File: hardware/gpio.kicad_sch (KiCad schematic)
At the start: 23 parts, among them J2 HDMI_C_1.3, U3 ECP5U_12_CABGA256, U5 PCA9306DC1

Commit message: Add a revision
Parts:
- R16, R18: JLCPCB Part # C25117 -> C25117
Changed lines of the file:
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@@
 			)
 		)
-		(property "JLCPCB Part #" "C25117 "
+		(property "JLCPCB Part #" "C25117"
 			(at 184.15 109.22 0)
 			(effects
@@
 			)
 		)
-		(property "JLCPCB Part #" "C25117 "
+		(property "JLCPCB Part #" "C25117"
 			(at 184.15 93.98 0)
 			(effects

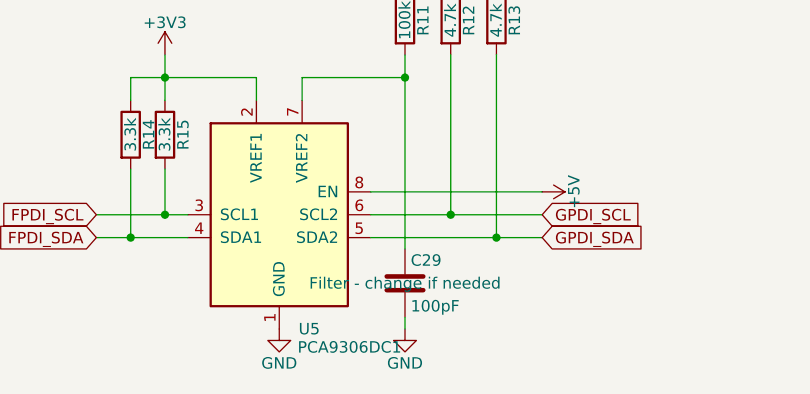
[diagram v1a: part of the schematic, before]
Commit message: Pre-prod fixes
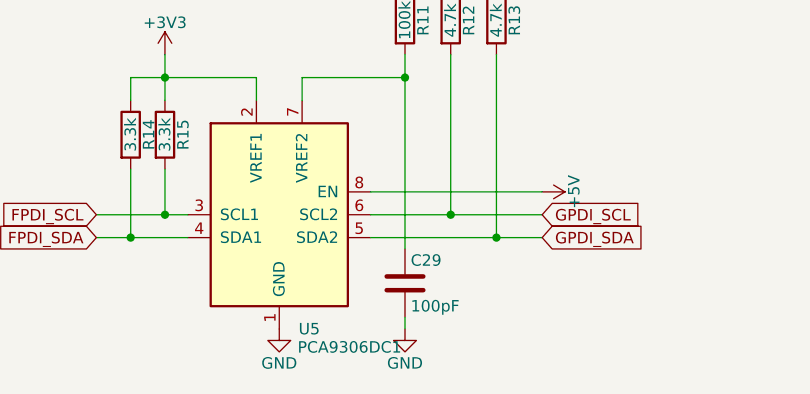
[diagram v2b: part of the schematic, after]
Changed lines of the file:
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@@
 					(size 1.27 1.27)
 				)
+				(hide yes)
 			)
 		)
@@
 		(on_board yes)
 		(dnp no)
-		(fields_autoplaced yes)
 		(property "Reference" "U3"
 			(at 104.14 97.7899 0)

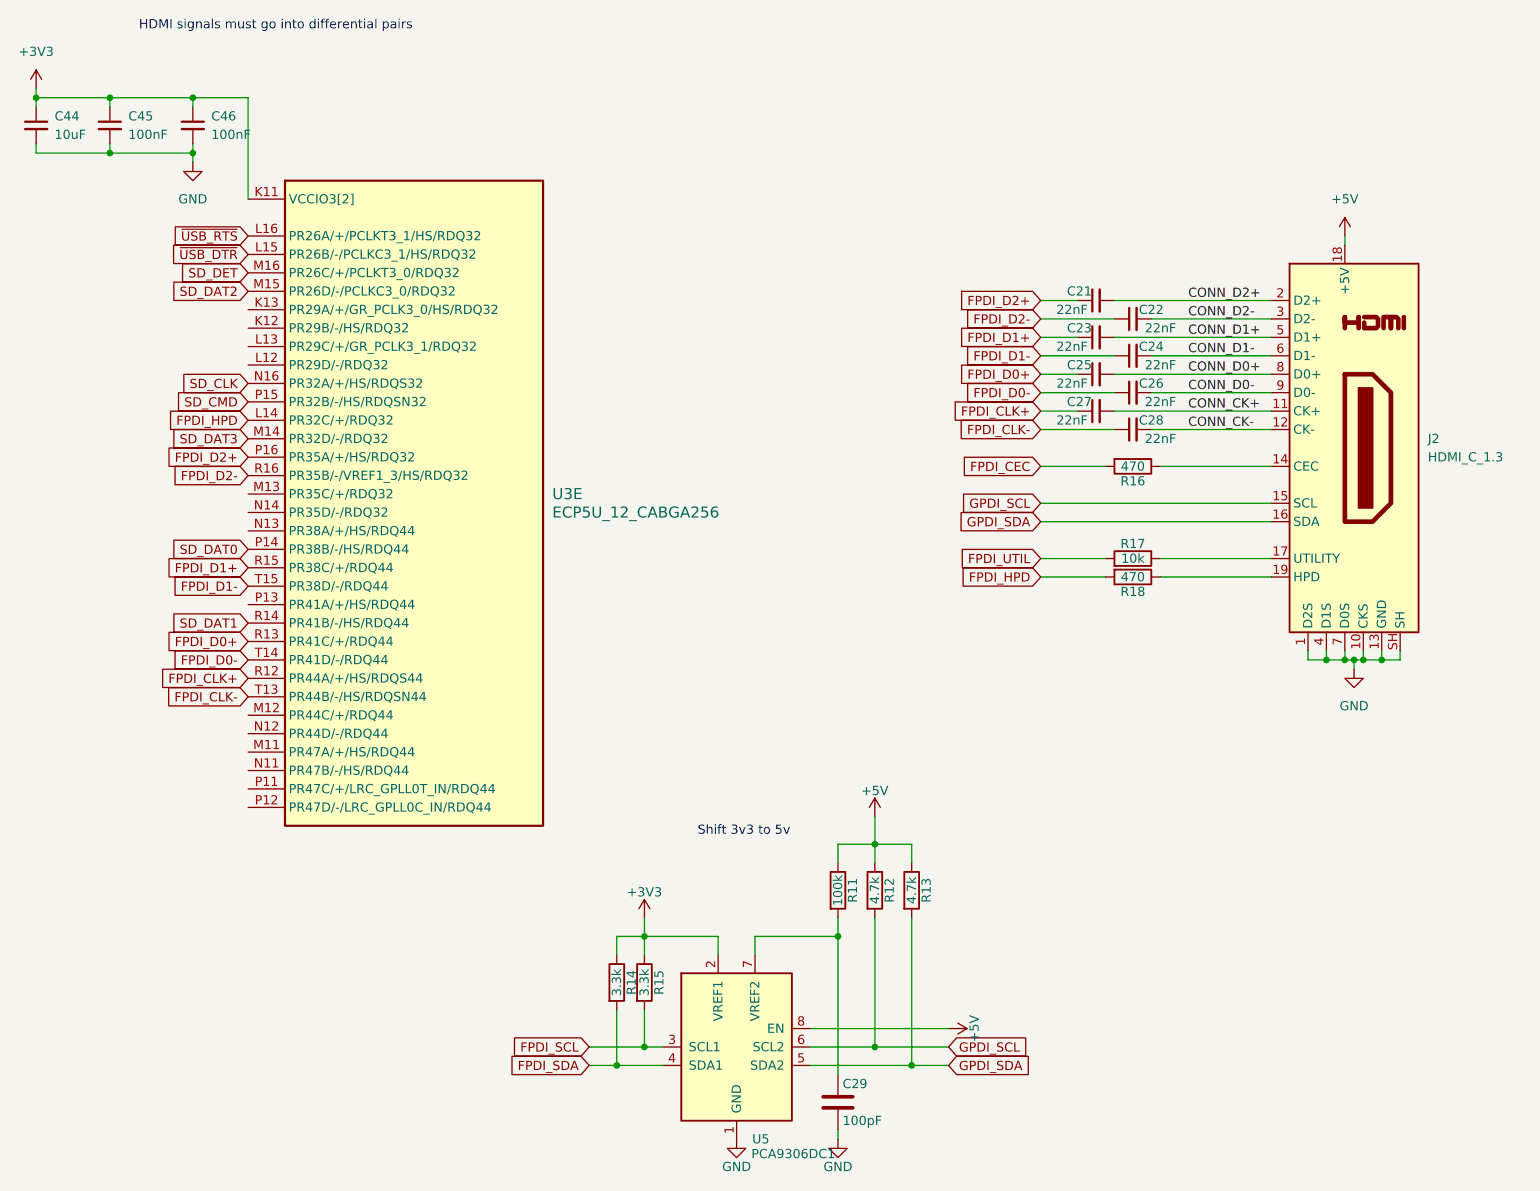
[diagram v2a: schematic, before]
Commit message: Final revision
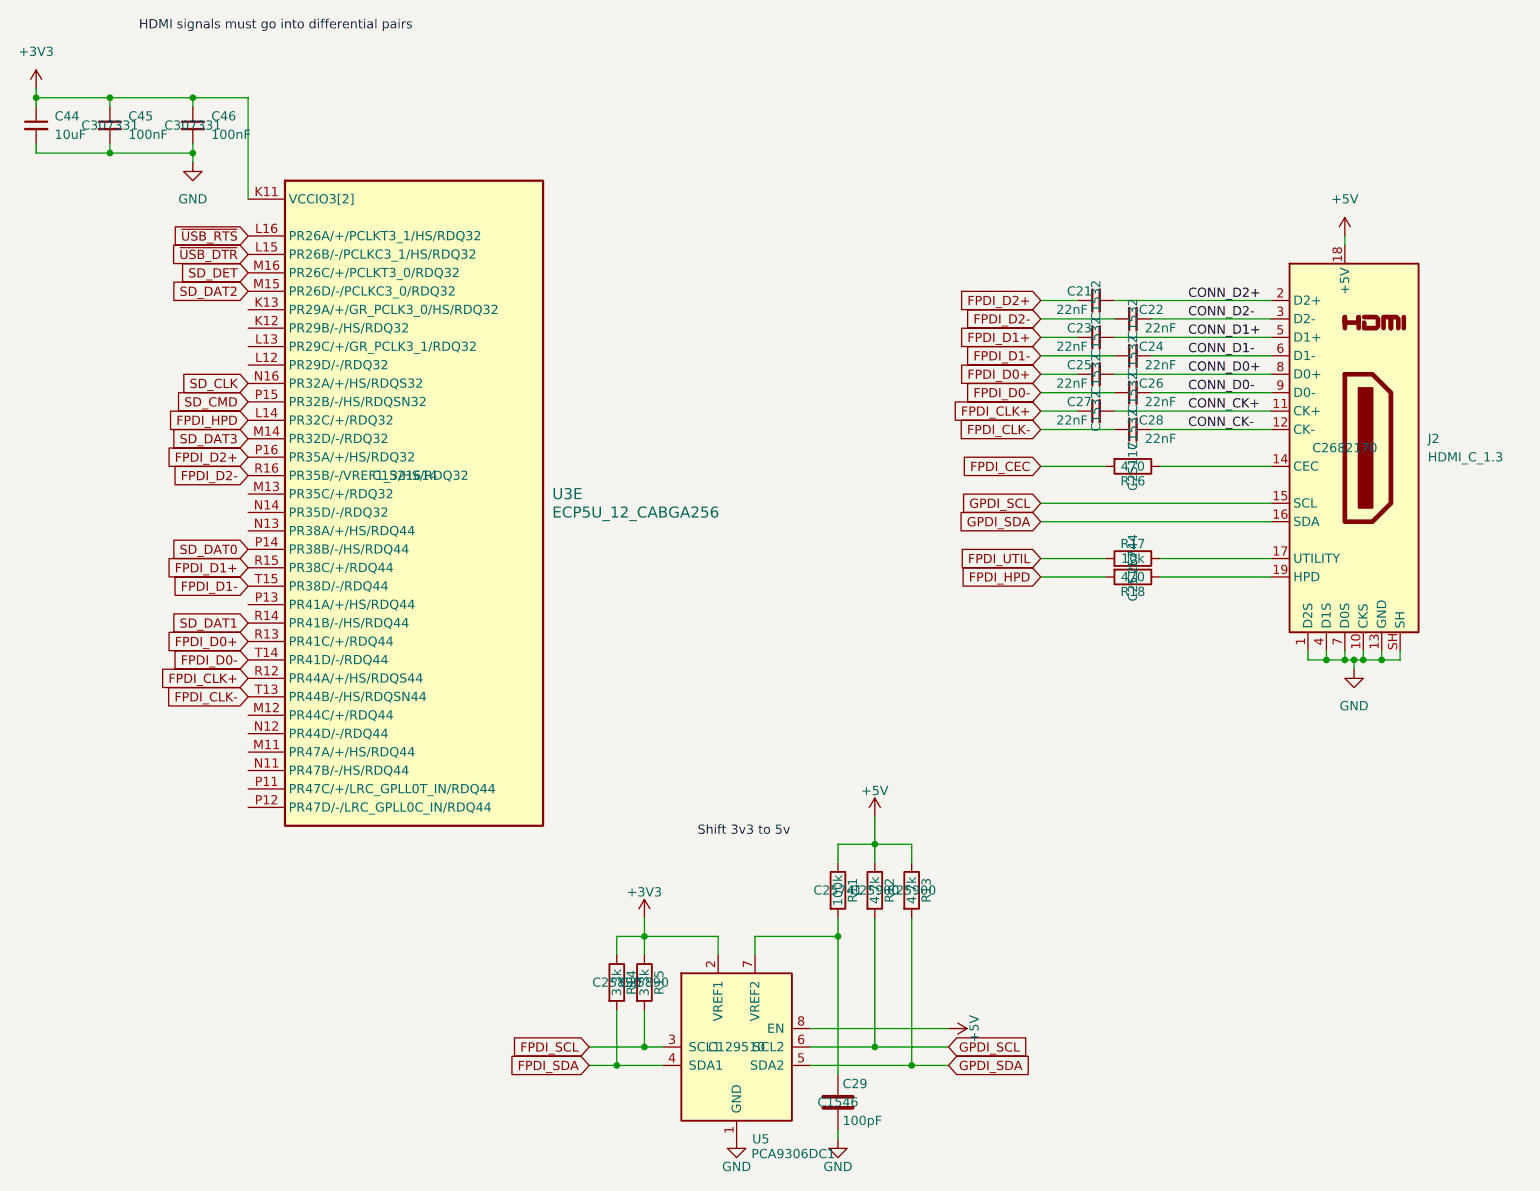
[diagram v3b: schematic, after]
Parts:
- C21, C22, C23, C24, C25, C26, C27, C28: JLCPCB Part # C1532 -> (none); LCSC Part # (none) -> C1532
- C29: JLCPCB Part # C1546 -> (none); LCSC Part # (none) -> C1546
- C45, C46: JLCPCB Part # C307331 -> (none); LCSC Part # (none) -> C307331
- J2: JLCPCB Part # C2682170 -> (none); LCSC Part # (none) -> C2682170
- R11: JLCPCB Part # C25741 -> (none); LCSC Part # (none) -> C25741
- R12, R13: JLCPCB Part # C25900 -> (none); LCSC Part # (none) -> C25900
- R14, R15: JLCPCB Part # C25890 -> (none); LCSC Part # (none) -> C25890
- R16, R18: JLCPCB Part # C25117 -> (none); LCSC Part # (none) -> C25117
- R17: JLCPCB Part # C25744 -> (none); LCSC Part # (none) -> C25744
- U3: JLCPCB Part # C1521614 -> (none); LCSC Part # (none) -> C1521614
- U5: JLCPCB Part # C129510 -> (none); LCSC Part # (none) -> C129510
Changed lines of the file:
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@@
 			)
 		)
-		(property "JLCPCB Part #" "C25741"
+		(property "LCSC Part #" "C25741"
 			(at 143.51 152.4 0)
 			(effects
@@
 					(size 1.27 1.27)
 				)
-				(hide yes)
 			)
 		)
@@
 			)
 		)
-		(property "JLCPCB Part #" "C25900 "
+		(property "LCSC Part #" "C25900 "
 			(at 148.59 152.4 0)
 			(effects
@@
 					(size 1.27 1.27)
 				)
-				(hide yes)
 			)
 		)
@@
 			)
 		)
-		(property "JLCPCB Part #" "C25900 "
+		(property "LCSC Part #" "C25900 "
 			(at 153.67 152.4 0)
 			(effects
@@
 					(size 1.27 1.27)
 				)
-				(hide yes)
 			)
 		)
@@
 			)
 		)
-		(property "JLCPCB Part #" "C1546 "
+		(property "LCSC Part #" "C1546 "
 			(at 143.51 181.61 0)
 			(effects
@@
 					(size 1.27 1.27)
 				)
-				(hide yes)
 			)
 		)
@@
 			)
 		)
-		(property "JLCPCB Part #" "C25890 "
+		(property "LCSC Part #" "C25890 "
 			(at 116.84 165.1 0)
 			(effects
@@
 					(size 1.27 1.27)
 				)
-				(hide yes)
 			)
 		)
@@
 			)
 		)
-		(property "JLCPCB Part #" "C25890 "
+		(property "LCSC Part #" "C25890 "
 			(at 113.03 165.1 0)
 			(effects
@@
 					(size 1.27 1.27)
 				)
-				(hide yes)
 			)
 		)
@@
 			)
 		)
-		(property "JLCPCB Part #" "C25117"
+		(property "LCSC Part #" "C25117"
 			(at 184.15 109.22 0)
 			(effects
@@
 					(size 1.27 1.27)
 				)
-				(hide yes)
 			)
 		)
@@
 			)
 		)
-		(property "JLCPCB Part #" "C1532"
+		(property "LCSC Part #" "C1532"
 			(at 179.07 81.28 0)
 			(effects
@@
 					(size 1.27 1.27)
 				)
-				(hide yes)
 			)
 		)
@@
 			)
 		)
-		(property "JLCPCB Part #" "C1532"
+		(property "LCSC Part #" "C1532"
 			(at 179.07 76.2 0)
 			(effects
@@
 					(size 1.27 1.27)
 				)
-				(hide yes)
 			)
 		)
@@
 			)
 		)
-		(property "JLCPCB Part #" "C307331 "
+		(property "LCSC Part #" "C307331 "
 			(at 54.61 46.99 0)
 			(effects
@@
 					(size 1.27 1.27)
 				)
-				(hide yes)
 			)
 		)
@@
 			)
 		)
-		(property "JLCPCB Part #" "C25117"
+		(property "LCSC Part #" "C25117"
 			(at 184.15 93.98 0)
 			(effects
@@
 					(size 1.27 1.27)
 				)
-				(hide yes)
 			)
 		)
@@
 			)
 		)
-		(property "JLCPCB Part #" "C1532"
+		(property "LCSC Part #" "C1532"
 			(at 184.15 83.82 0)
 			(effects
@@
 					(size 1.27 1.27)
 				)
-				(hide yes)
 			)
 		)
@@
 			)
 		)
-		(property "JLCPCB Part #" "C307331 "
+		(property "LCSC Part #" "C307331 "
 			(at 43.18 46.99 0)
 			(effects
@@
 					(size 1.27 1.27)
 				)
-				(hide yes)
 			)
 		)
@@
 			)
 		)
-		(property "JLCPCB Part #" "C1532"
+		(property "LCSC Part #" "C1532"
 			(at 184.15 88.9 0)
 			(effects
@@
 					(size 1.27 1.27)
 				)
-				(hide yes)
 			)
 		)
@@
 			)
 		)
-		(property "JLCPCB Part #" "C1532"
+		(property "LCSC Part #" "C1532"
 			(at 184.15 78.74 0)
 			(effects
@@
 					(size 1.27 1.27)
 				)
-				(hide yes)
 			)
 		)
@@
 			)
 		)
-		(property "JLCPCB Part #" "C1521614"
+		(property "LCSC Part #" "C1521614"
 			(at 83.82 95.25 0)
 			(effects
@@
 					(size 1.27 1.27)
 				)
-				(hide yes)
 			)
 		)
@@
 			)
 		)
-		(property "JLCPCB Part #" "C25744"
+		(property "LCSC Part #" "C25744"
 			(at 184.15 106.68 0)
 			(effects
@@
 					(size 1.27 1.27)
 				)
-				(hide yes)
 			)
 		)
@@
 			)
 		)
-		(property "JLCPCB Part #" "C1532"
+		(property "LCSC Part #" "C1532"
 			(at 179.07 71.12 0)
 			(effects
@@
 					(size 1.27 1.27)
 				)
-				(hide yes)
 			)
 		)
@@
 			)
 		)
-		(property "JLCPCB Part #" "C129510"
+		(property "LCSC Part #" "C129510"
 			(at 129.54 173.99 0)
 			(effects
@@
 					(size 1.27 1.27)
 				)
-				(hide yes)
 			)
 		)
@@
 			)
 		)
-		(property "JLCPCB Part #" "C2682170"
+		(property "LCSC Part #" "C2682170"
 			(at 213.36 91.44 0)
 			(effects
@@
 					(size 1.27 1.27)
 				)
-				(hide yes)
 			)
 		)
@@
 			)
 		)
-		(property "JLCPCB Part #" "C1532"
+		(property "LCSC Part #" "C1532"
 			(at 184.15 73.66 0)
 			(effects
@@
 					(size 1.27 1.27)
 				)
-				(hide yes)
 			)
 		)
@@
 			)
 		)
-		(property "JLCPCB Part #" "C1532"
+		(property "LCSC Part #" "C1532"
 			(at 179.07 86.36 0)
 			(effects
@@
 					(size 1.27 1.27)
 				)
-				(hide yes)
-			)
-		)
+			)
+		)
